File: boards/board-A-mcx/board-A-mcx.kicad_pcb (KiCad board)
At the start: 4 copper layers, 74.8 x 137.1 mm, 30 parts, among them J5 SAMTEC_QSE-040-01-X-D-A, K0 Samtec_MCX-J-P-H-RA-TH1, K1 Samtec_MCX-J-P-H-RA-TH1, K10 Samtec_MCX-J-P-H-RA-TH1, K11 Samtec_MCX-J-P-H-RA-TH1, K12 Samtec_MCX-J-P-H-RA-TH1, K13 Samtec_MCX-J-P-H-RA-TH1, K14 Samtec_MCX-J-P-H-RA-TH1, K15 Samtec_MCX-J-P-H-RA-TH1, K16 Samtec_MCX-J-P-H-RA-TH1, K17 Samtec_MCX-J-P-H-RA-TH1, K18 Samtec_MCX-J-P-H-RA-TH1, K19 Samtec_MCX-J-P-H-RA-TH1, K2 Samtec_MCX-J-P-H-RA-TH1, K20 Samtec_MCX-J-P-H-RA-TH1, K21 Samtec_MCX-J-P-H-RA-TH1, K22 Samtec_MCX-J-P-H-RA-TH1, K23 Samtec_MCX-J-P-H-RA-TH1, K3 Samtec_MCX-J-P-H-RA-TH1, K4 Samtec_MCX-J-P-H-RA-TH1, K5 Samtec_MCX-J-P-H-RA-TH1, K6 Samtec_MCX-J-P-H-RA-TH1, K7 Samtec_MCX-J-P-H-RA-TH1, K8 Samtec_MCX-J-P-H-RA-TH1, K9 Samtec_MCX-J-P-H-RA-TH1

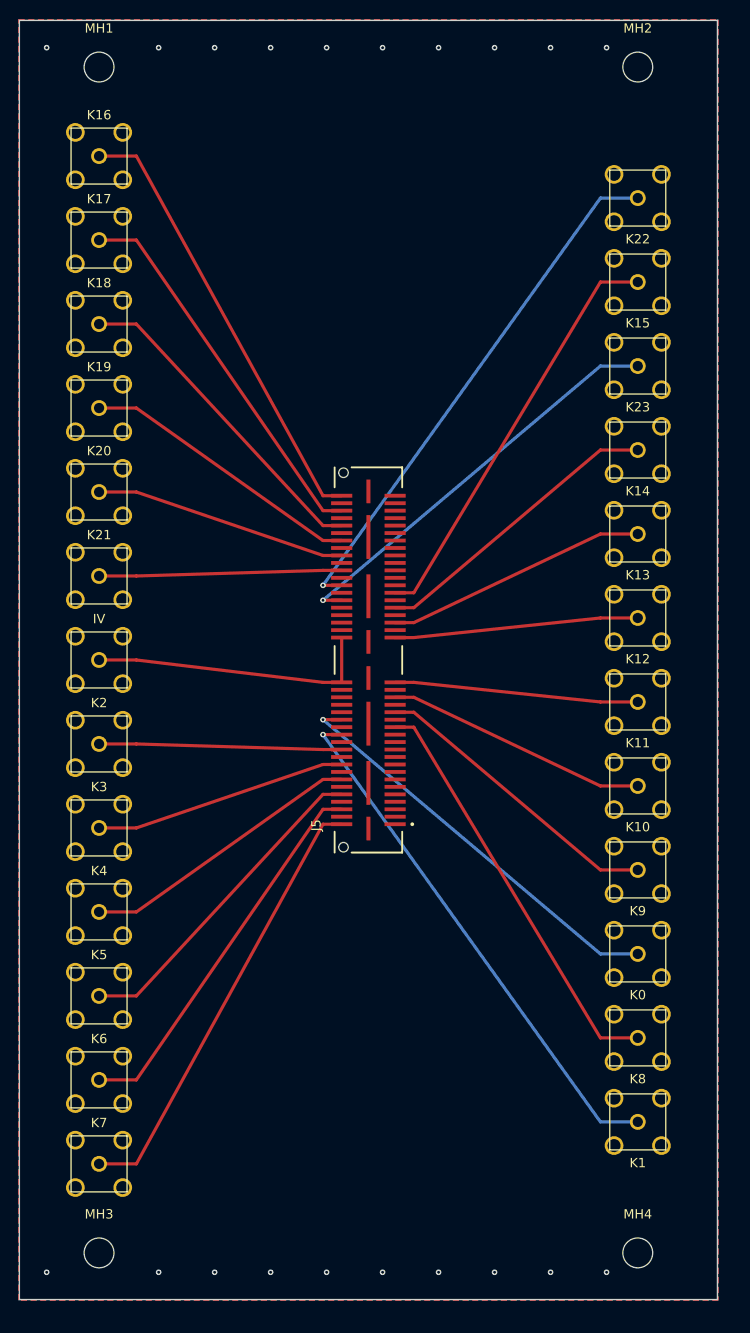
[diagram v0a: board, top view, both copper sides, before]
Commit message: initial upload
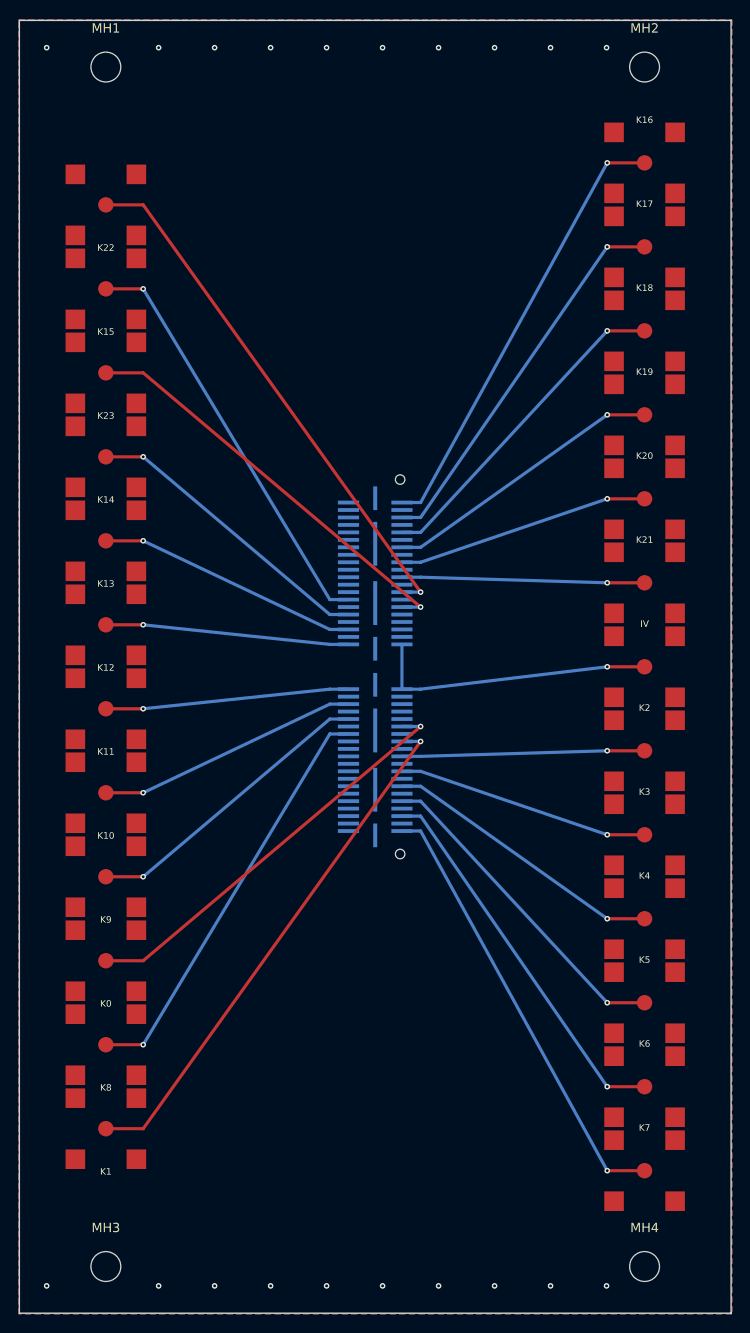
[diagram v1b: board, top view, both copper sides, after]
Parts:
- removed the IV at (17.5, 78.5)
- added IV: Samtec_MCX-J-P-X-ST-SM1, Samtec_MCX-J-P-X-ST-SM1, F.Cu at (76.0, 79.3)
- J5: moved to B.Cu
- K0, K1, K10, K11, K12, K13, K14, K15, K16, K17, K18, K19, K2, K20, K21, K22, K23, K3, K4, K5, K6, K7, K8, K9: value Samtec_MCX-J-P-H-RA-TH1 -> Samtec_MCX-J-P-X-ST-SM1; footprint Samtec_MCX-J-P-H-RA-TH1 -> Samtec_MCX-J-P-X-ST-SM1
- moved K16 58.5 mm to (76.0, 25.3)
- moved K17 58.5 mm to (76.0, 34.3)
- moved K18 58.5 mm to (76.0, 43.3)
- moved K19 58.5 mm to (76.0, 52.3)
- moved K2 58.5 mm to (76.0, 88.3)
- moved K20 58.5 mm to (76.0, 61.3)
- moved K21 58.5 mm to (76.0, 70.3)
- moved K3 58.5 mm to (76.0, 97.3)
- moved K4 58.5 mm to (76.0, 106.3)
- moved K5 58.5 mm to (76.0, 115.3)
- moved K6 58.5 mm to (76.0, 124.3)
- moved K7 58.5 mm to (76.0, 133.3)
- moved K0 57.0 mm to (18.3, 110.8)
- moved K1 57.0 mm to (18.3, 128.8)
- moved K10 57.0 mm to (18.3, 92.8)
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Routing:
- net SIPM_K12: vias 0 -> 1
- net SIPM_K8: vias 0 -> 1
- net SIPM_K7: vias 0 -> 1
- net SIPM_K5: vias 0 -> 1
- net SIPM_K15: vias 0 -> 1
- net SIPM_K14: vias 0 -> 1
- net SIPM_K9: vias 0 -> 1
- net SIPM_K16: vias 0 -> 1
- net SIPM_K13: vias 0 -> 1
- net SIPM_K11: vias 0 -> 1
- net SIPM_K10: vias 0 -> 1
- net SIPM_K3: vias 0 -> 1
- net SIPM_K21: vias 0 -> 1
- net SIPM_K20: vias 0 -> 1
- net SIPM_K2: vias 0 -> 1
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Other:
- board size 74.8 x 137.1 mm -> 76.3 x 138.5 mm
